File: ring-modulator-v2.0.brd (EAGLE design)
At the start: 34.3 x 24.1 mm, 27 parts, among them IC1 TL072D, U1 MC1496DR2G

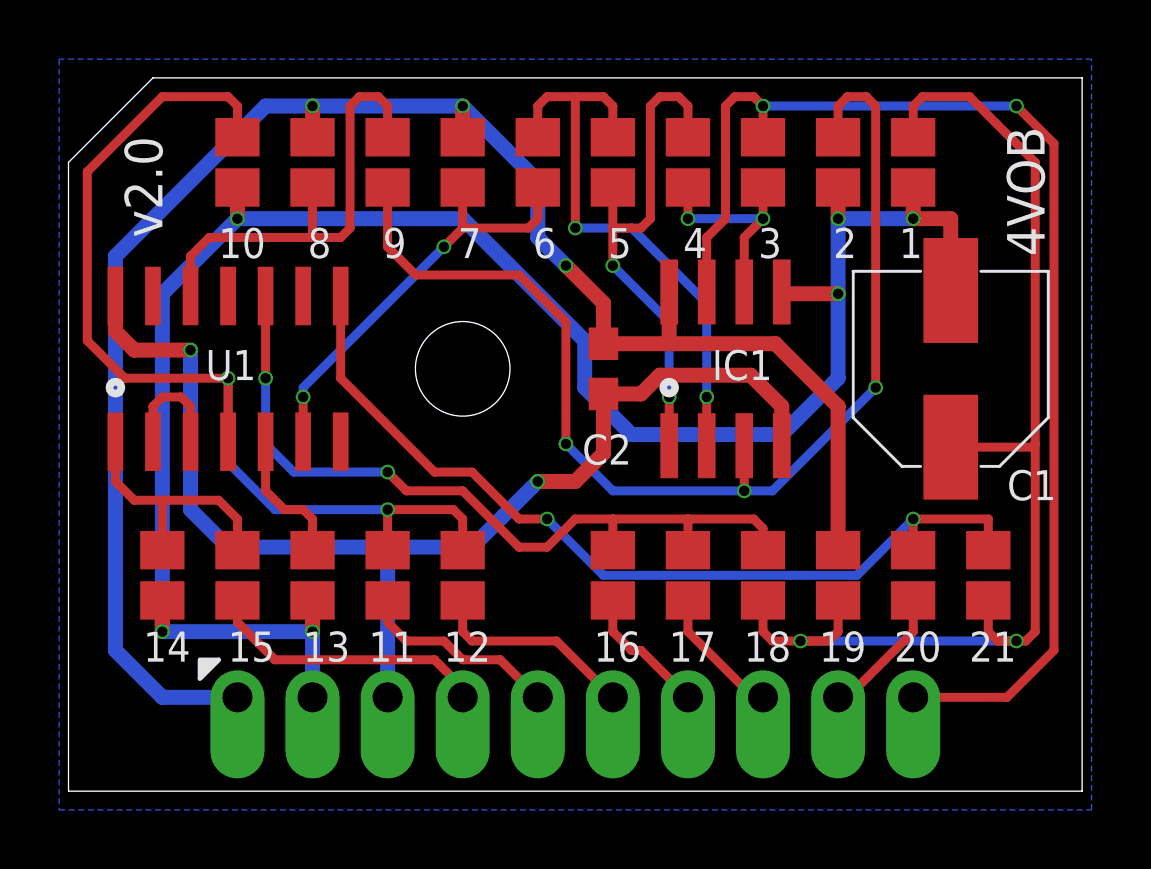
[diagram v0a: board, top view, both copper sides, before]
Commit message: moving
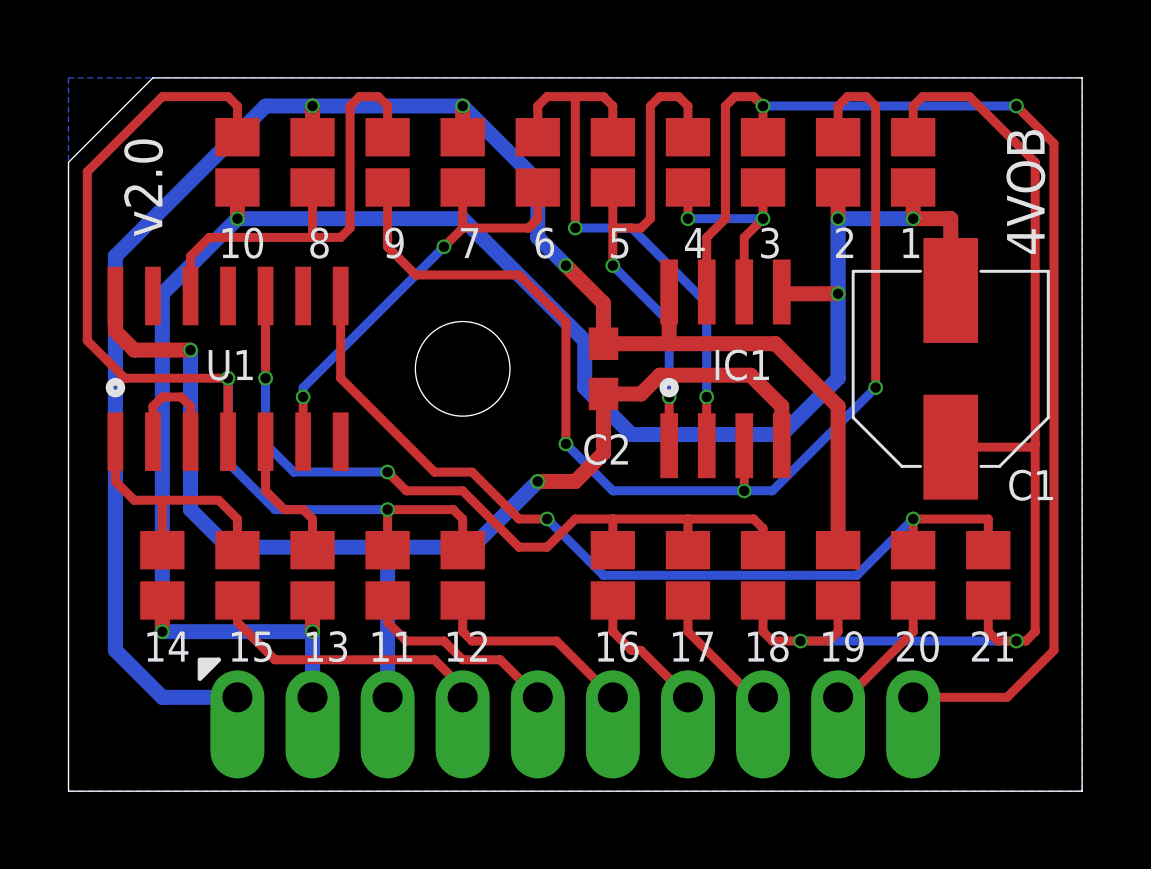
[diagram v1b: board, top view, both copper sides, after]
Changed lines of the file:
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@@
 <wire x1="28.575" y1="19.3675" x2="26.035" y2="19.3675" width="0.508" layer="16"/>
 <polygon width="0.3048" layer="16">
-<vertex x="34.6075" y="24.765"/>
-<vertex x="-0.3175" y="24.765"/>
-<vertex x="-0.3175" y="-0.635"/>
-<vertex x="34.6075" y="-0.635"/>
+<vertex x="34.29" y="24.13"/>
+<vertex x="0" y="24.13"/>
+<vertex x="0" y="0"/>
+<vertex x="34.29" y="0"/>
 </polygon>
 </signal>
